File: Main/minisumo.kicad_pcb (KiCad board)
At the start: 4 copper layers, 80 x 36.5 mm, 53 parts, among them J10 SDER, J11 PDER, J2 M_DER, J3 USB, J4 M_IZ, J7 SIZQ, J8 SFRE, J9 PIZQ, SW1 ACT, SW2 SW_DIP_x02, SW3 EN, SW4 BOOT, SW6 SW_Nidec_CAS-120A1, U2 AMS1117-3.3, U3 TA6586, U4 ESP-WROOM-32, U5 TA6586, U6 Mini360

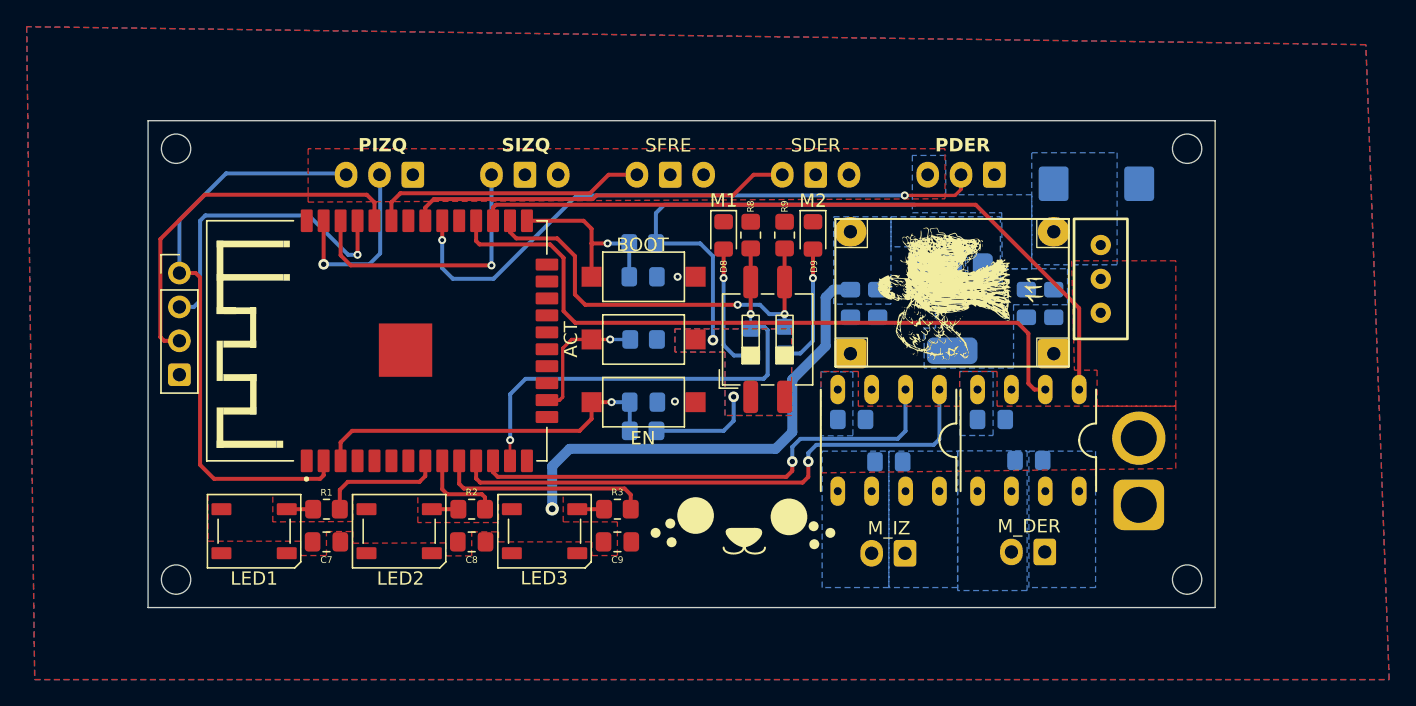
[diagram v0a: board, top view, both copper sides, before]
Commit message: .
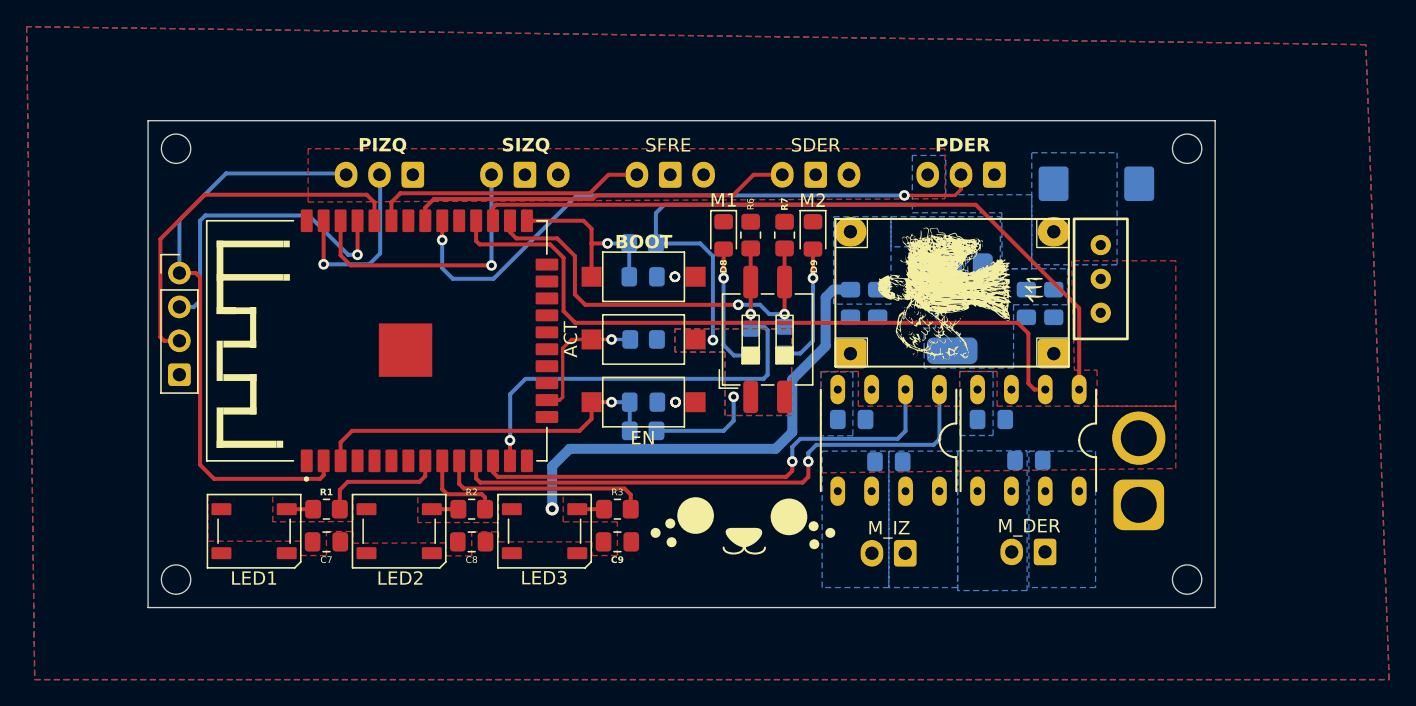
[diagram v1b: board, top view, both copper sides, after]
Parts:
- renumbered R12 to R10, R6 to R4, R7 to R5, R8 to R6, R9 to R7, R10 to R8, R11 to R9
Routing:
- net GND: vias 2 -> 4
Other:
- board text added: "CE2=100uF CE3-4=1uF C=100nF R1-5=330 R6-10=10K"
- board text removed: "CE2=100uF CE3-4=1uF C=100nF R1-7=330 R8-11=10K"
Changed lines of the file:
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@@
 				(font
 					(size 0.5 0.5)
-					(thickness 0.125)
+					(thickness 0.1)
+					(bold yes)
 				)
 			)
@@
 		)
 		(property "Value" "BOOT"
-			(at 0.075 2.4 0)
+			(at 0 2.6 0)
 			(layer "F.SilkS")
 			(effects
 				(font
 					(size 1 1)
-					(thickness 0.125)
+					(thickness 0.2)
+					(bold yes)
 				)
 			)
@@
 				(font
 					(size 0.5 0.5)
-					(thickness 0.125)
+					(thickness 0.1)
+					(bold yes)
 				)
 			)
@@
 				(font
 					(size 0.5 0.5)
-					(thickness 0.125)
+					(thickness 0.1)
+					(bold yes)
 				)
 			)
@@
 		(descr "Resistor SMD 0805 (2012 Metric), square (rectangular) end terminal, IPC-7351 nominal with elongated pad for handsoldering. (Body size source: IPC-SM-782 page 72, https://www.pcb-3d.com/wordpress/wp-content/uploads/ipc-sm-782a_amendment_1_and_2.pdf), generated with kicad-footprint-generator")
 		(tags "resistor handsolder")
-		(property "Reference" "R8"
-			(at 2.15 -0.005 90)
+		(property "Reference" "R6"
+			(at 2.325 -0.005 90)
 			(layer "F.SilkS")
 			(effects
@@
 		(descr "Resistor SMD 0805 (2012 Metric), square (rectangular) end terminal, IPC-7351 nominal with elongated pad for handsoldering. (Body size source: IPC-SM-782 page 72, https://www.pcb-3d.com/wordpress/wp-content/uploads/ipc-sm-782a_amendment_1_and_2.pdf), generated with kicad-footprint-generator")
 		(tags "resistor handsolder")
-		(property "Reference" "R9"
-			(at 2.15 0 90)
+		(property "Reference" "R7"
+			(at 2.325 0 90)
 			(layer "F.SilkS")
 			(effects
 				(font
 					(size 0.5 0.5)
-					(thickness 0.125)
+					(thickness 0.1)
+					(bold yes)
 				)
 			)
@@
 		(tags "resistor handsolder")
 		(property "Reference" "R1"
-			(at 0 -1.65 0)
+			(at 0 1.275 0)
 			(layer "F.SilkS")
-			(hide yes)
 			(effects
 				(font
-					(size 1 1)
-					(thickness 0.15)
+					(size 0.5 0.5)
+					(thickness 0.125)
+					(bold yes)
 				)
 			)
@@
 			(layer "F.Fab")
 		)
-		(fp_text user "${REFERENCE}"
-			(at 0 1.25 0)
-			(layer "F.SilkS")
-			(effects
-				(font
-					(size 0.5 0.5)
-					(thickness 0.08)
-				)
-			)
-		)
 		(pad "1" smd roundrect
 			(at -1 0 180)
@@
 		(tags "capacitor handsolder")
 		(property "Reference" "C6"
-			(at 0.0125 -1.15 90)
+			(at 0.05 -1.25 90)
 			(layer "B.SilkS")
 			(effects
@@
 		(descr "Resistor SMD 0805 (2012 Metric), square (rectangular) end terminal, IPC-7351 nominal with elongated pad for handsoldering. (Body size source: IPC-SM-782 page 72, https://www.pcb-3d.com/wordpress/wp-content/uploads/ipc-sm-782a_amendment_1_and_2.pdf), generated with kicad-footprint-generator")
 		(tags "resistor handsolder")
-		(property "Reference" "R10"
+		(property "Reference" "R8"
 			(at 0 -1.35 0)
 			(layer "B.SilkS")
@@
 		(tags "capacitor tantalum")
 		(property "Reference" "CE2"
-			(at -1 0.575 0)
+			(at 0.05 -2.725 0)
 			(layer "B.SilkS")
 			(effects
 				(font
 					(size 0.5 0.5)
-					(thickness 0.125)
+					(thickness 0.1)
+					(bold yes)
 				)
 				(justify mirror)
@@
 		(tags "capacitor handsolder")
 		(property "Reference" "CE4"
-			(at -0.8125 -1.45 90)
+			(at 0 1.15 90)
 			(layer "B.SilkS")
 			(effects
@@
 		(descr "Resistor SMD 0805 (2012 Metric), square (rectangular) end terminal, IPC-7351 nominal with elongated pad for handsoldering. (Body size source: IPC-SM-782 page 72, https://www.pcb-3d.com/wordpress/wp-content/uploads/ipc-sm-782a_amendment_1_and_2.pdf), generated with kicad-footprint-generator")
 		(tags "resistor handsolder")
-		(property "Reference" "R7"
+		(property "Reference" "R5"
 			(at 0 -1.155 90)
 			(layer "B.SilkS")
@@
 		(descr "Resistor SMD 0805 (2012 Metric), square (rectangular) end terminal, IPC-7351 nominal with elongated pad for handsoldering. (Body size source: IPC-SM-782 page 72, https://www.pcb-3d.com/wordpress/wp-content/uploads/ipc-sm-782a_amendment_1_and_2.pdf), generated with kicad-footprint-generator")
 		(tags "resistor handsolder")
-		(property "Reference" "R11"
+		(property "Reference" "R9"
 			(at 0 1.325 0)
 			(layer "B.SilkS")
@@
 		(descr "Resistor SMD 0805 (2012 Metric), square (rectangular) end terminal, IPC-7351 nominal with elongated pad for handsoldering. (Body size source: IPC-SM-782 page 72, https://www.pcb-3d.com/wordpress/wp-content/uploads/ipc-sm-782a_amendment_1_and_2.pdf), generated with kicad-footprint-generator")
 		(tags "resistor handsolder")
-		(property "Reference" "R6"
+		(property "Reference" "R4"
 			(at 0 -1.22 90)
 			(layer "B.SilkS")
@@
 	(footprint "Connector_JST:JST_XH_B2B-XH-A_1x02_P2.50mm_Vertical"
 		(layer "B.Cu")
-		(at 215.9775 88.73 180)
+		(at 215.9975 88.73 180)
 		(descr "JST XH series connector, B2B-XH-A (http://www.jst-mfg.com/product/pdf/eng/eXH.pdf), generated with kicad-footprint-generator")
 		(tags "connector JST XH vertical")
@@
 	(footprint "Connector_JST:JST_XH_B2B-XH-A_1x02_P2.50mm_Vertical"
 		(layer "B.Cu")
-		(at 205.4975 88.83 180)
+		(at 205.5175 88.83 180)
 		(descr "JST XH series connector, B2B-XH-A (http://www.jst-mfg.com/product/pdf/eng/eXH.pdf), generated with kicad-footprint-generator")
 		(tags "connector JST XH vertical")
@@
 		(tags "capacitor handsolder")
 		(property "Reference" "C5"
-			(at -0.0125 -1.175 90)
+			(at 0 -1.2 90)
 			(layer "B.SilkS")
 			(effects
@@
 		(descr "Resistor SMD 0805 (2012 Metric), square (rectangular) end terminal, IPC-7351 nominal with elongated pad for handsoldering. (Body size source: IPC-SM-782 page 72, https://www.pcb-3d.com/wordpress/wp-content/uploads/ipc-sm-782a_amendment_1_and_2.pdf), generated with kicad-footprint-generator")
 		(tags "resistor handsolder")
-		(property "Reference" "R12"
+		(property "Reference" "R10"
 			(at 0 1.15 0)
 			(layer "B.SilkS")
@@
 		)
 	)
-	(gr_text "CE2=100uF\nCE3-4=1uF\nC=100nF\nR1-7=330\nR8-11=10K\n"
-		(at 199.525 79.575 0)
+	(gr_text "CE2=100uF\nCE3-4=1uF\nC=100nF\nR1-5=330\nR6-10=10K\n"
+		(at 199 86.25 0)
 		(layer "B.SilkS")
 		(effects
@@
 	)
 	(via
-		(at 188.45 68.1)
-		(size 0.6)
-		(drill 0.3)
+		(at 188.25 68.1)
+		(size 0.8)
+		(drill 0.4)
 		(layers "F.Cu" "B.Cu")
+		(free yes)
 		(net 1)
 	)
 	(via
-		(at 188.25 77.45)
-		(size 0.6)
-		(drill 0.3)
+		(at 188.3 77.5)
+		(size 0.8)
+		(drill 0.4)
+		(layers "F.Cu" "B.Cu")
+		(free yes)
+		(net 1)
+	)
+	(via
+		(at 188.3 77.5)
+		(size 0.8)
+		(drill 0.4)
+		(layers "F.Cu" "B.Cu")
+		(free yes)
+		(net 1)
+	)
+	(via
+		(at 188.25 68.1)
+		(size 0.8)
+		(drill 0.4)
 		(layers "F.Cu" "B.Cu")
 		(free yes)
@@
 	(via
 		(at 183.5 77.5)
-		(size 0.6)
-		(drill 0.3)
+		(size 0.8)
+		(drill 0.4)
 		(layers "F.Cu" "B.Cu")
 		(net 2)
@@
 	(via
 		(at 183.2 65.6)
-		(size 0.6)
-		(drill 0.3)
+		(size 0.8)
+		(drill 0.4)
 		(layers "F.Cu" "B.Cu")
 		(net 5)
@@
 	)
 	(via
-		(at 164.455 66.45)
-		(size 0.6)
-		(drill 0.3)
+		(at 164.45 66.45)
+		(size 0.8)
+		(drill 0.4)
 		(layers "F.Cu" "B.Cu")
 		(net 6)
@@
 	(segment
 		(start 164.5 66.45)
+		(end 164.45 66.45)
+		(width 0.3)
+		(layer "B.Cu")
+		(net 6)
+	)
+	(segment
+		(start 164.45 66.45)
 		(end 163.75 66.45)
 		(width 0.3)
@@
 	(via
 		(at 174.5 67.25)
-		(size 0.6)
-		(drill 0.3)
+		(size 0.8)
+		(drill 0.4)
 		(layers "F.Cu" "B.Cu")
 		(net 17)
@@
 	)
 	(segment
-		(start 170.805 63.9)
-		(end 170.805 65.345)
-		(width 0.3)
-		(layer "F.Cu")
-		(net 32)
-	)
-	(segment
 		(start 170.805 65.345)
 		(end 170.8 65.35)
@@
 	)
 	(segment
+		(start 170.805 65.545)
+		(end 170.805 65.345)
+		(width 0.3)
+		(layer "F.Cu")
+		(net 32)
+	)
+	(segment
 		(start 205.476 62)
 		(end 209.25 62)
@@
 		(net 32)
 	)
+	(segment
+		(start 170.805 63.9)
+		(end 170.805 65.545)
+		(width 0.3)
+		(layer "F.Cu")
+		(net 32)
+	)
 	(via
-		(at 205.476 62)
-		(size 0.6)
-		(drill 0.3)
+		(at 205.45 62)
+		(size 0.8)
+		(drill 0.4)
 		(layers "F.Cu" "B.Cu")
 		(net 32)
 	)
 	(via
-		(at 170.8 65.35)
-		(size 0.6)
-		(drill 0.3)
+		(at 170.805 65.345)
+		(size 0.8)
+		(drill 0.4)
 		(layers "F.Cu" "B.Cu")
 		(net 32)
@@
 	(segment
 		(start 205.476 62)
-		(end 180.9 62)
+		(end 205.45 62)
 		(width 0.3)
 		(layer "B.Cu")
@@
 	)
 	(segment
+		(start 205.45 62)
+		(end 180.9 62)
+		(width 0.3)
+		(layer "B.Cu")
+		(net 32)
+	)
+	(segment
 		(start 214.75 72.35)
 		(end 213.95 71.55)
@@
 	)
 	(segment
-		(start 191.9 68.25)
+		(start 191.9 68.2)
 		(end 191.9 66.025)
 		(width 0.3)
@@
 		(net 36)
 	)
+	(segment
+		(start 191.9 68.25)
+		(end 191.9 68.2)
+		(width 0.3)
+		(layer "F.Cu")
+		(net 36)
+	)
 	(via
 		(at 191.9 68.2)
-		(size 0.6)
-		(drill 0.3)
+		(size 0.8)
+		(drill 0.4)
 		(layers "F.Cu" "B.Cu")
 		(net 36)
@@
 	(via
 		(at 198.6 68.2)
-		(size 0.6)
-		(drill 0.3)
+		(size 0.8)
+		(drill 0.4)
 		(layers "F.Cu" "B.Cu")
 		(net 37)
@@
 	)
 	(via
-		(at 183.4 72.8)
-		(size 0.6)
-		(drill 0.3)
+		(at 183.5 72.8)
+		(size 0.8)
+		(drill 0.4)
 		(layers "F.Cu" "B.Cu")
 		(net 40)
@@
 		(start 175.885 81.9)
 		(end 175.885 80.365)
-		(width 0.2)
+		(width 0.3)
 		(layer "F.Cu")
 		(net 50)
@@
 	)
 	(via
-		(at 175.9 80.35)
-		(size 0.6)
-		(drill 0.3)
+		(at 175.885 80.365)
+		(size 0.8)
+		(drill 0.4)
 		(layers "F.Cu" "B.Cu")
 		(net 50)
@@
 	(via
 		(at 193.93 70.9)
-		(size 0.6)
-		(drill 0.3)
+		(size 0.8)
+		(drill 0.4)
 		(layers "F.Cu" "B.Cu")
 		(net 50)
@@
 	)
 	(via
-		(at 192.95 70.2)
-		(size 0.6)
-		(drill 0.3)
+		(at 193 70.2)
+		(size 0.8)
+		(drill 0.4)
 		(layers "F.Cu" "B.Cu")
 		(net 51)
@@
 	(via
 		(at 196.47 70.9)
-		(size 0.6)
-		(drill 0.3)
+		(size 0.8)
+		(drill 0.4)
 		(layers "F.Cu" "B.Cu")
 		(net 51)
 	)
 	(segment
+		(start 193 70.2)
+		(end 194.625 70.2)
+		(width 0.3)
+		(layer "B.Cu")
+		(net 51)
+	)
+	(segment
 		(start 195.325 70.9)
 		(end 196.47 70.9)
@@
 	(segment
 		(start 192.95 70.2)
-		(end 194.625 70.2)
+		(end 193 70.2)
 		(width 0.3)
 		(layer "B.Cu")
